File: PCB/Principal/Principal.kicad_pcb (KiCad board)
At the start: 2 copper layers, 17 parts, among them J1 STM32_P1, J2 STM32_P2, J3 Sensor_Golpes, J4 Teclado, J5 Sensor_Unidades, J6 Display_16x2, J7 Lector_RFID, J8 IN_Alimentación

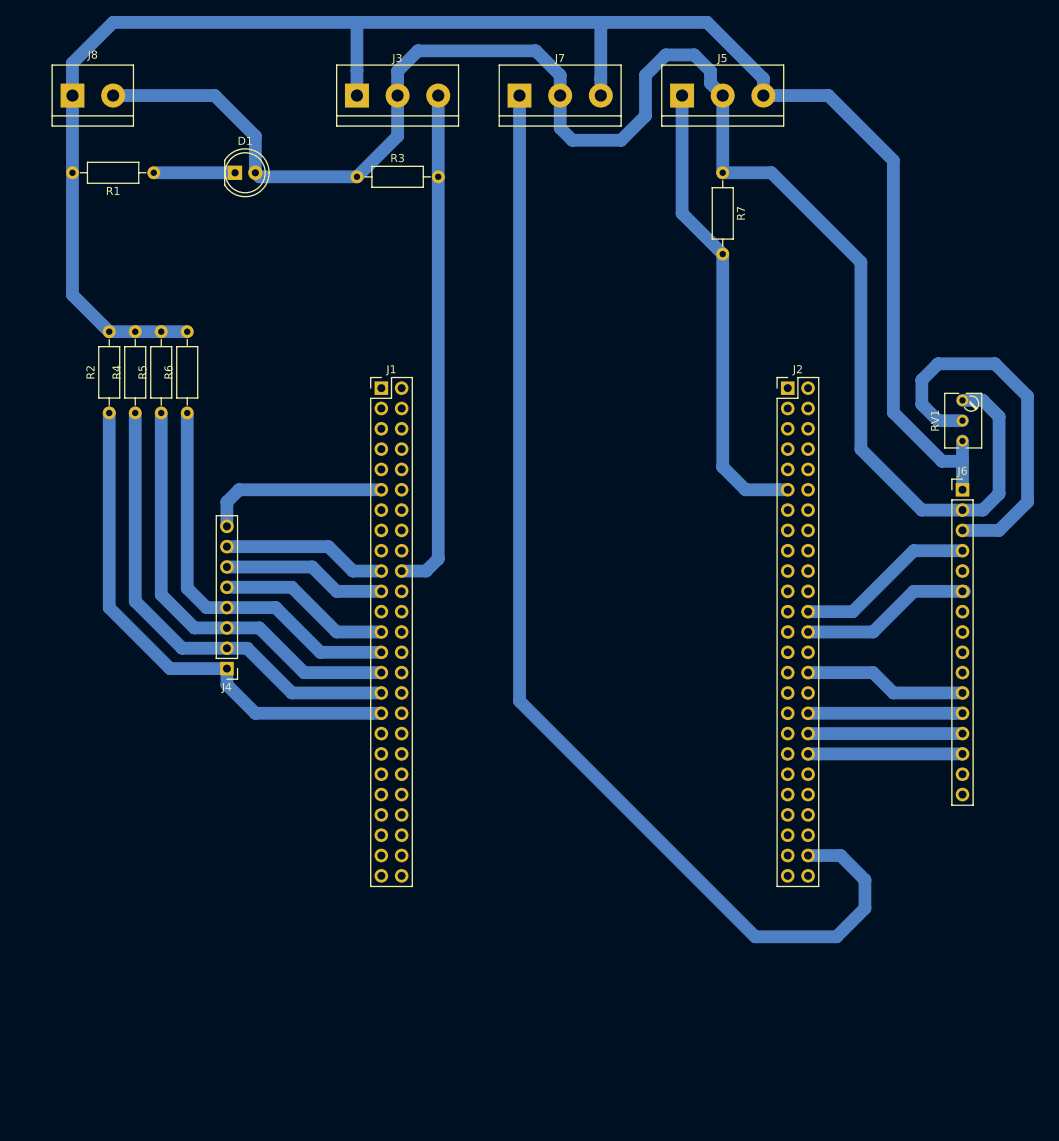
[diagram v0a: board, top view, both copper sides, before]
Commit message: ALTA PLACA GUACHO
Nada, eso.
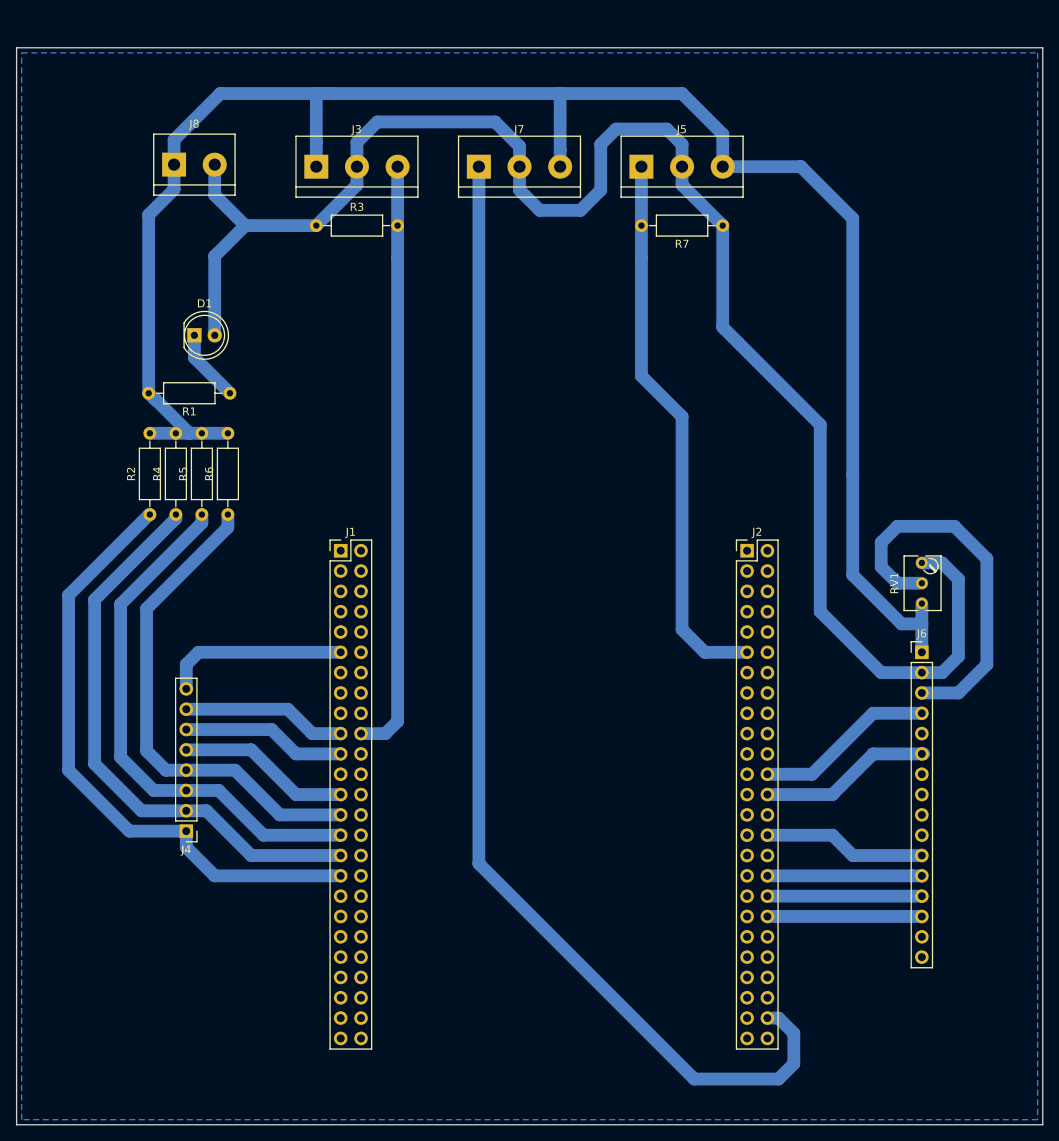
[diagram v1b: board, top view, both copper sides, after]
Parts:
- moved R1 29.2 mm to (108.6, 61.6)
- moved J6 20.9 mm to (195.1, 94.0)
- moved D1 20.9 mm to (104.1, 54.4)
- moved J1 20.9 mm to (122.4, 81.3)
- moved J2 20.9 mm to (173.2, 81.3)
- moved RV1 20.9 mm to (195.1, 82.8)
- moved J4 20.9 mm to (103.1, 116.3)
- moved J8 15.4 mm to (101.6, 33.0)
- moved R2 13.7 mm to (98.6, 76.8)
- moved R4 13.7 mm to (101.8, 76.8)
- moved R5 13.7 mm to (105.1, 76.8)
- moved R6 13.7 mm to (108.3, 76.8)
- moved J7 10.2 mm to (139.7, 33.3)
- moved J3 10.2 mm to (119.4, 33.3)
- moved J5 10.2 mm to (160.0, 33.3)
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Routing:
- net Net-(J1-Pad33): track 65.1 -> 76.9 mm
- net Net-(J1-Pad31): track 59.0 -> 70.9 mm
- net Net-(J1-Pad29): track 54.3 -> 66.1 mm
- net Net-(J1-Pad27): track 49.5 -> 61.3 mm
- net Net-(J2-Pad11): track 57.8 -> 69.3 mm
- net Net-(J1-Pad20): track 63.1 -> 74.5 mm
- net GND: track 225.4 -> 228.0 mm
- net Net-(J2-Pad48): track 144.5 -> 146.3 mm
- net +5V: track 204.5 -> 205.6 mm
- net Net-(D1-Pad1): track 10.2 -> 9.08 mm
- added copper zone on B.Cu, net GND
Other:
- board outline added: 128.3 x 134.6 mm
